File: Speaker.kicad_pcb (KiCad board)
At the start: 4 copper layers, 26 parts, among them J1 AudioJack3_Ground, J2 Screw_Terminal_01x02, U1 NE5532, U2 NE5532

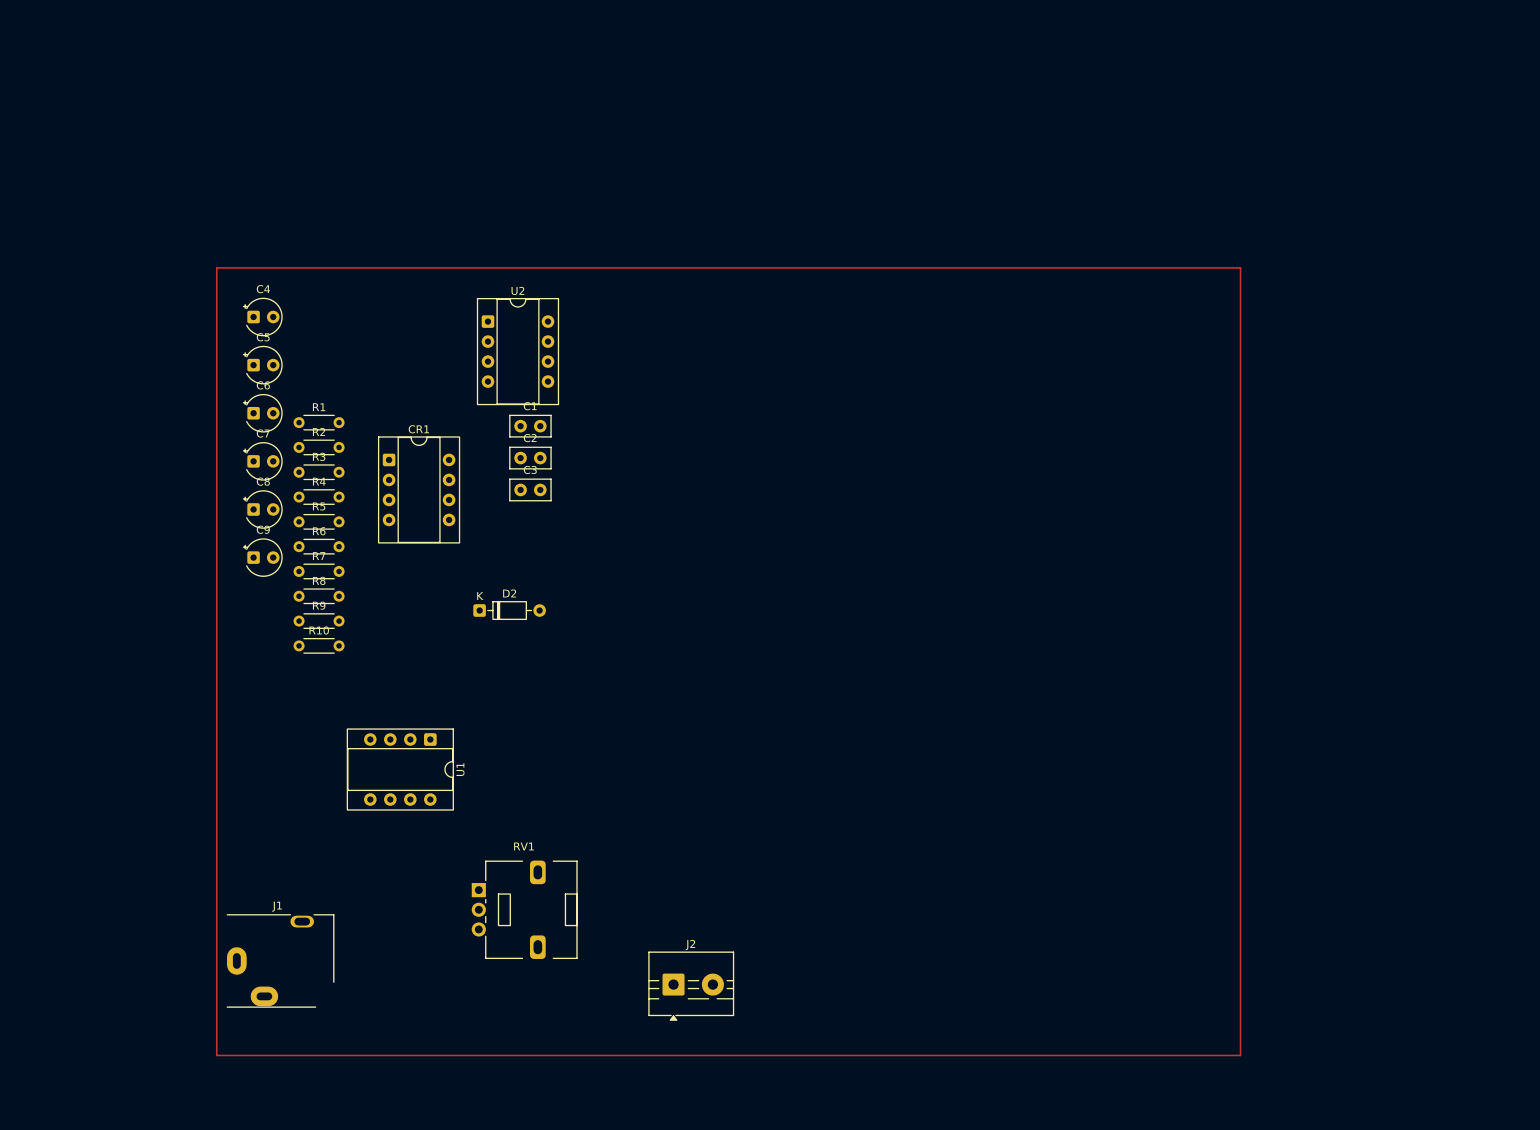
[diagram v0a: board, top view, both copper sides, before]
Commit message: Created PCB
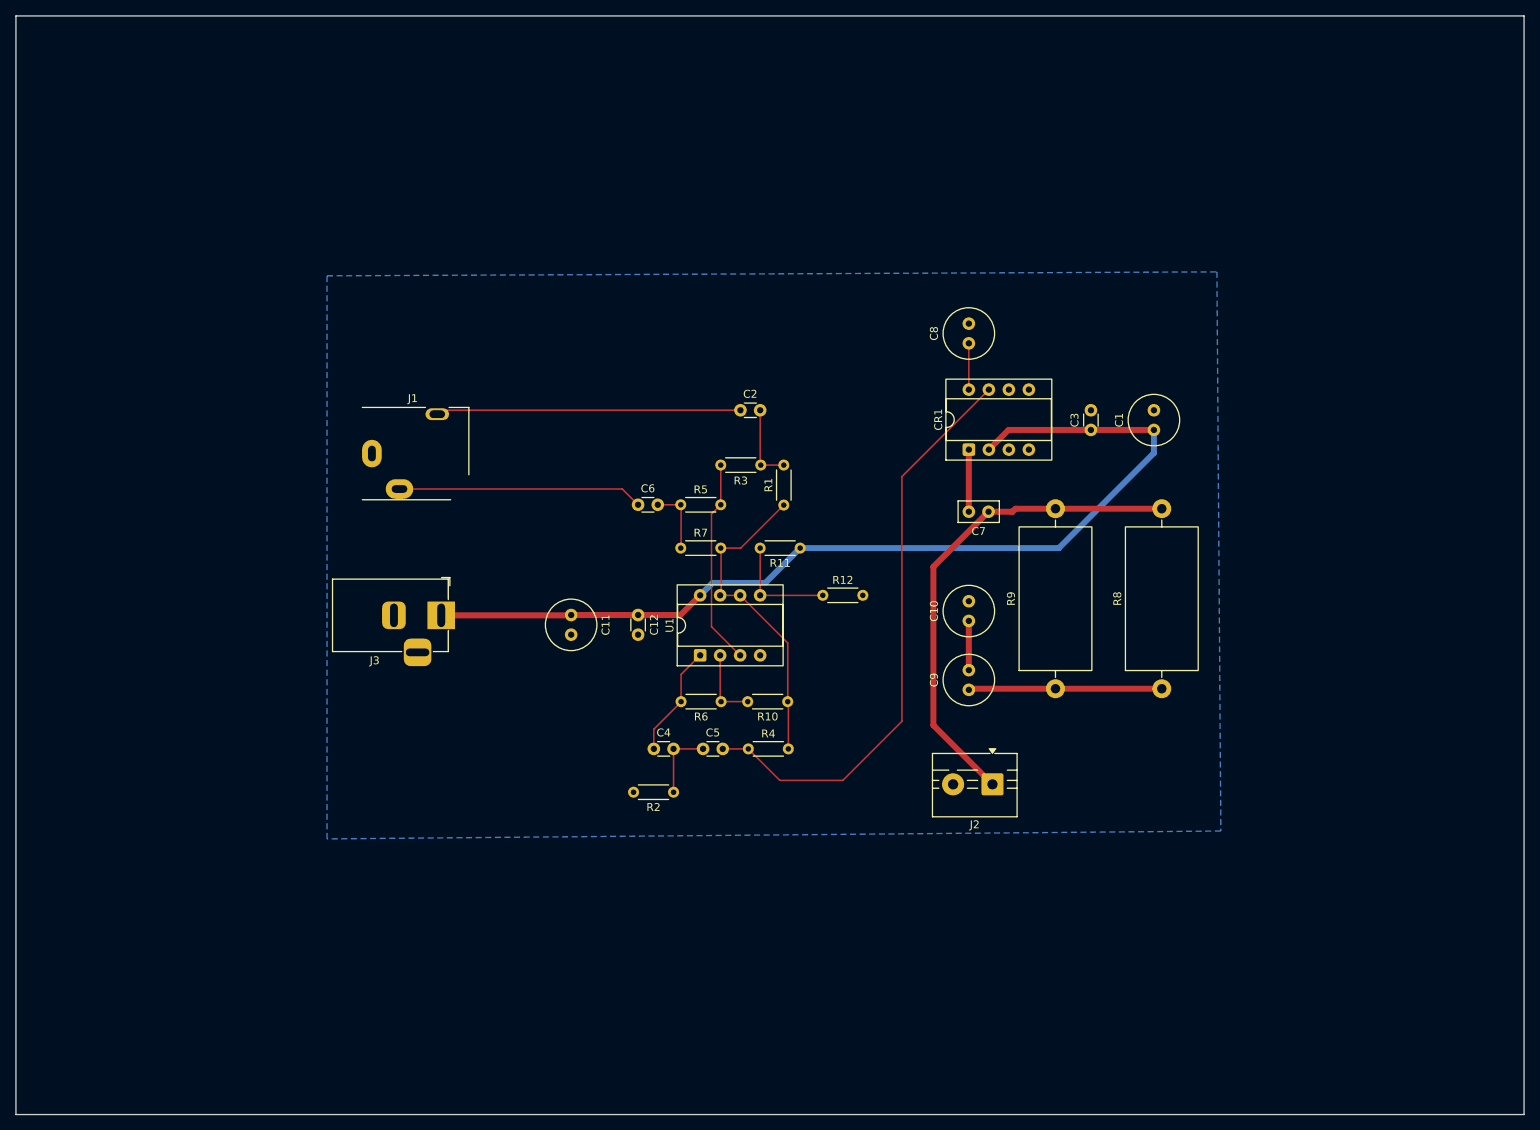
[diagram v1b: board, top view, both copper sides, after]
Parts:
- removed D2: D_Zener, Diode_THT:D_DO-35_SOD27_P7.62mm_Horizontal
- removed RV1: R_Potentiometer_US, Potentiometer_THT:Potentiometer_Alps_RK09L_Single_Vertical
- removed U2: NE5532, Package_DIP:CERDIP-8_W7.62mm_SideBrazed_Socket
- added C10: 10uF, Capacitor_THT:C_Radial_D6.3mm_H5.0mm_P2.50mm, F.Cu at (184.5, 90.3)
- added C11: 10uF, Capacitor_THT:C_Radial_D6.3mm_H5.0mm_P2.50mm, F.Cu at (134.0, 89.6)
- added C12: 100nF, Capacitor_THT:C_Disc_D3.0mm_W1.6mm_P2.50mm, F.Cu at (142.5, 89.6)
- added J3: Barrel_Jack_MountingPin, Connector_BarrelJack:BarrelJack_Horizontal, F.Cu at (117.5, 89.6)
- added R11: r=100K, Resistor_THT:R_Axial_DIN0204_L3.6mm_D1.6mm_P5.08mm_Horizontal, F.Cu at (163.1, 81.1)
- added R12: r=100K, Resistor_THT:R_Axial_DIN0204_L3.6mm_D1.6mm_P5.08mm_Horizontal, F.Cu at (166.0, 87.1)
- C1: value 100nF -> 10uF; footprint Capacitor_THT:C_Disc_D5.0mm_W2.5mm_P2.50mm -> Capacitor_THT:C_Radial_D6.3mm_H5.0mm_P2.50mm
- C2, C3: footprint Capacitor_THT:C_Disc_D5.0mm_W2.5mm_P2.50mm -> Capacitor_THT:C_Disc_D3.0mm_W1.6mm_P2.50mm
- C4, C5, C6: value 10uF -> 100nF; footprint Capacitor_THT:CP_Radial_Tantal_D4.5mm_P2.50mm -> Capacitor_THT:C_Disc_D3.0mm_W1.6mm_P2.50mm
- C7: value 10uF -> 200uF; footprint Capacitor_THT:CP_Radial_Tantal_D4.5mm_P2.50mm -> Capacitor_THT:C_Disc_D5.0mm_W2.5mm_P2.50mm
- C8: value 10nF -> 100uF; footprint Capacitor_THT:CP_Radial_Tantal_D4.5mm_P2.50mm -> Capacitor_THT:C_Radial_D6.3mm_H5.0mm_P2.50mm
- C9: footprint Capacitor_THT:CP_Radial_Tantal_D4.5mm_P2.50mm -> Capacitor_THT:C_Radial_D6.3mm_H5.0mm_P2.50mm
- J1: value AudioJack3_Ground -> AudioJack3
- R10, R5: value r=4.7 -> r=50K
- R4, R7: value r=50K -> r=10K
- R6: value r=10K -> r=50K
- R8: value r=50K -> r=10; footprint Resistor_THT:R_Axial_DIN0204_L3.6mm_D1.6mm_P5.08mm_Horizontal -> Resistor_THT:R_Axial_DIN0918_L18.0mm_D9.0mm_P22.86mm_Horizontal
- R9: value r=600 -> r=10; footprint Resistor_THT:R_Axial_DIN0204_L3.6mm_D1.6mm_P5.08mm_Horizontal -> Resistor_THT:R_Axial_DIN0918_L18.0mm_D9.0mm_P22.86mm_Horizontal
- moved R8 110.2 mm to (209.0, 98.9), turned to 90 degrees
- moved R9 96.4 mm to (195.5, 98.9), turned to 90 degrees
- moved C7 93.5 mm to (187.0, 76.5), turned to 180 degrees
- moved C8 93.2 mm to (184.5, 55.1), turned to 90 degrees
- moved C9 92.4 mm to (184.5, 99.1), turned to 90 degrees
- moved C1 80.4 mm to (208.0, 66.1), turned to 90 degrees
- moved C5 75.0 mm to (150.8, 106.6)
- moved C4 74.8 mm to (144.5, 106.6)
- moved CR1 73.6 mm to (184.5, 68.6), turned to 90 degrees
- moved C3 72.8 mm to (200.0, 66.1), turned to 90 degrees
- moved J1 66.7 mm to (108.7, 69.1)
- moved R4 65.4 mm to (156.5, 106.6)
- moved R2 64.6 mm to (147.0, 112.1), turned to 180 degrees
- moved R10 62.5 mm to (161.5, 100.6), turned to 180 degrees
- moved R1 62.4 mm to (161.0, 75.6), turned to 90 degrees
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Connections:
- C1 pad 1: Net-(C1-Pad1) -> +9V
- C1 pad 2: Net-(C1-Pad2) -> GND
- C3 pad 1: Net-(C3-Pad1) -> +9V
- C3 pad 2: /PreAmp Out -> GND
- C4 pad 1: Net-(D2-K) -> Net-(C4-Pad1)
- C4 pad 2: GND -> /PreAmp Out
- C5 pad 1: GND -> /PreAmp Out
- C5 pad 2: +12V -> Net-(C5-Pad2)
- C6 pad 2: GND -> Net-(C6-Pad2)
- C7 pad 1: Net-(C7-Pad1) -> Net-(J2-Pin_1)
- C7 pad 2: GND -> Net-(CR1-OUT1)
- C8 pad 2: Net-(CR1-IN-2) -> GND
- C9 pad 1: Net-(CR1-IN-2) -> Net-(C9-Pad1)
- C9 pad 2: GND -> Net-(C10-Pad1)
- CR1 pad 2: +12V -> +9V
- CR1 pad 3: Net-(CR1-OUT2) -> unconnected-(CR1-OUT2-Pad3)
- CR1 pad 5: Net-(CR1-IN-2) -> GND
- CR1 pad 7: Net-(CR1-IN-1-Pad7) -> Net-(C5-Pad2)
- J1 pad R: Net-(C1-Pad1) -> Net-(C2-Pad1)
- J1 pad T: Net-(C2-Pad1) -> Net-(C6-Pad1)
- J2 pad 1: Net-(CR1-OUT2) -> Net-(J2-Pin_1)
- J2 pad 2: Net-(CR1-OUT1) -> GND
- R1 pad 2: Net-(C1-Pad2) -> Net-(C2-Pad2)
- R10 pad 1: Net-(CR1-OUT2) -> /VREF
- R10 pad 2: Net-(C6-Pad1) -> Net-(U1A--)
- R2 pad 1: Net-(C2-Pad2) -> /PreAmp Out
- R2 pad 2: /VREF -> GND
- R3 pad 1: Net-(C1-Pad2) -> Net-(C2-Pad2)
- R4 pad 1: Net-(C2-Pad2) -> Net-(C5-Pad2)
- R4 pad 2: Net-(U1A-+) -> /VREF
- R5 pad 1: Net-(CR1-OUT1) -> Net-(C6-Pad2)
- R5 pad 2: Net-(C7-Pad1) -> Net-(U1A-+)
- R6 pad 1: /PreAmp Out -> Net-(U1A--)
- R6 pad 2: GND -> Net-(C4-Pad1)
- R7 pad 1: Net-(U1A--) -> Net-(C6-Pad2)
- R7 pad 2: Net-(C3-Pad1) -> /VREF
- R8 pad 1: GND -> Net-(C9-Pad1)
- R8 pad 2: Net-(U1A--) -> Net-(J2-Pin_1)
- R9 pad 1: +12V -> Net-(C9-Pad1)
- R9 pad 2: Net-(D2-K) -> Net-(J2-Pin_1)
- U1 pad 1: Net-(C3-Pad1) -> Net-(C4-Pad1)
- U1 pad 4: (no net) -> GND
- U1 pad 5: (no net) -> Net-(U1B-+)
- U1 pad 6: (no net) -> /VREF
- U1 pad 7: (no net) -> /VREF
- U1 pad 8: (no net) -> +9V
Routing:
- net +9V: track 0.00 -> 124.0 mm
- net Net-(C5-Pad2): track 0.00 -> 74.2 mm
- net Net-(J2-Pin_1): track 0.00 -> 63.4 mm
- net /VREF: track 0.00 -> 40.9 mm
- net Net-(C2-Pad1): track 0.00 -> 38.7 mm
- net Net-(C6-Pad1): track 0.00 -> 31.1 mm
- net Net-(U1A-+): track 0.00 -> 26.2 mm
- net Net-(C9-Pad1): track 0.00 -> 24.6 mm
- net Net-(C4-Pad1): track 0.00 -> 14.3 mm
- net Net-(U1B-+): track 0.00 -> 14.0 mm
- net Net-(C2-Pad2): track 0.00 -> 9.91 mm
- net Net-(U1A--): track 0.00 -> 9.31 mm
- net /PreAmp Out: track 0.00 -> 9.25 mm
- net Net-(C6-Pad2): track 0.00 -> 8.44 mm
- net Net-(CR1-OUT1): track 0.00 -> 7.88 mm
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- added copper zone on B.Cu, net GND
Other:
- board outline added: 191.5 x 139.5 mm
- copper layers 4 -> 2
